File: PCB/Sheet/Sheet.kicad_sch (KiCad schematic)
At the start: 15 parts, among them U1 MCP9700Ax-ELT, U2 MCP2562-E-MF, U3 ATtiny1616-M, U6 MCP2515-xST

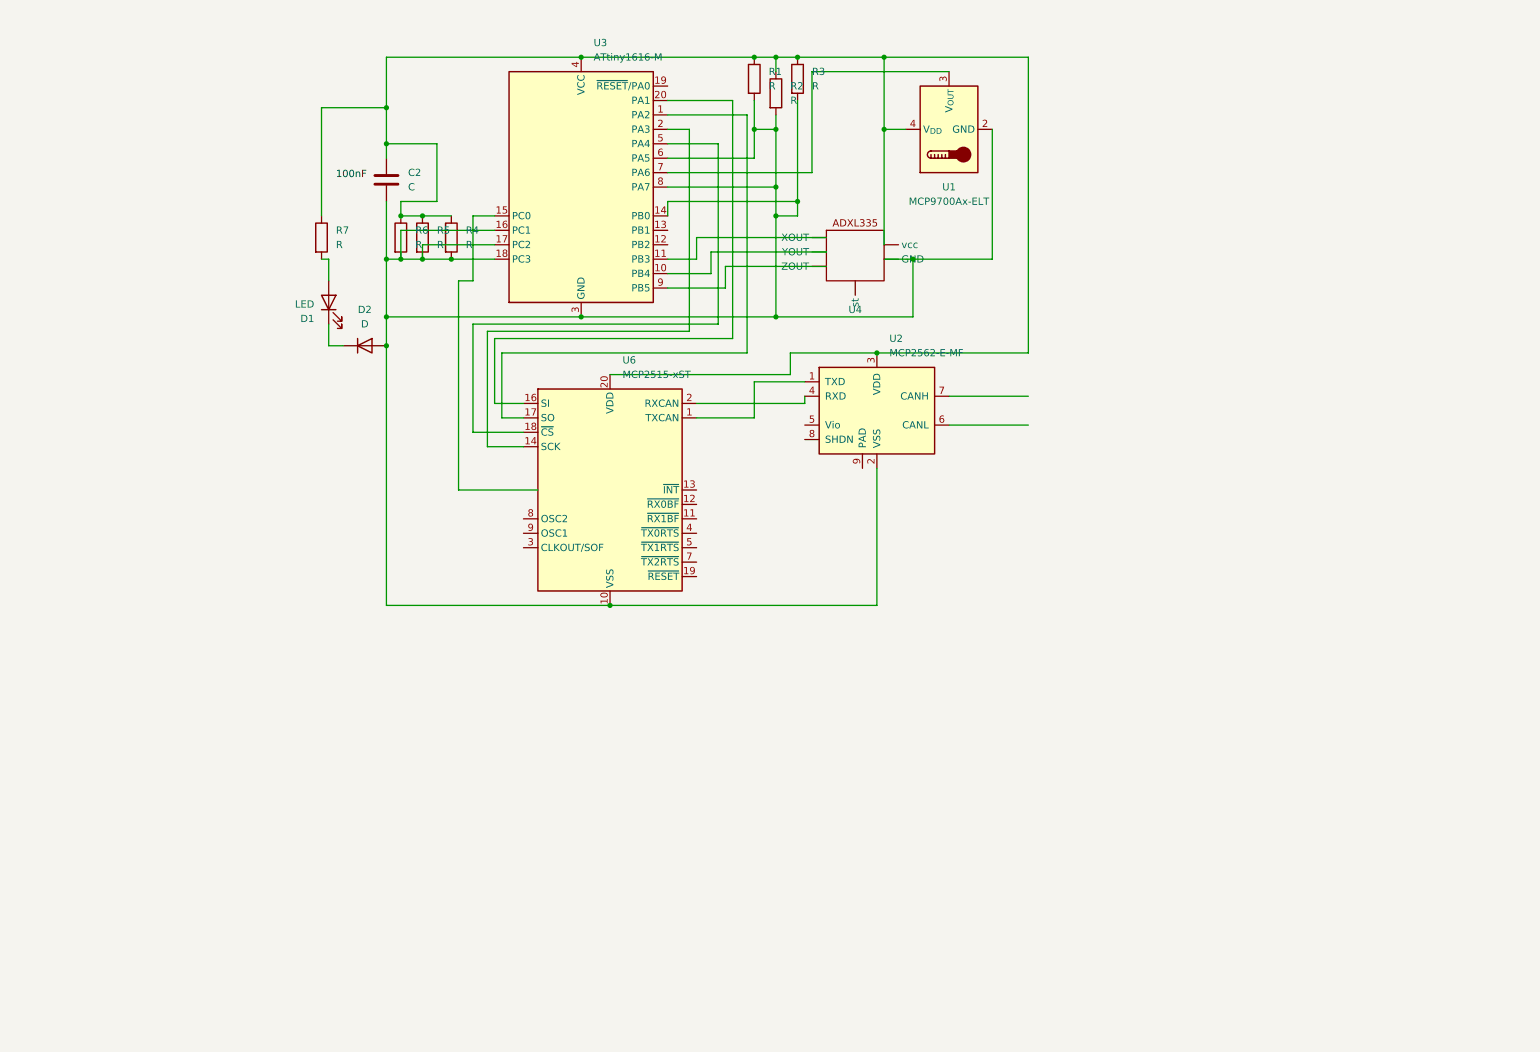
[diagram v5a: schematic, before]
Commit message: updates
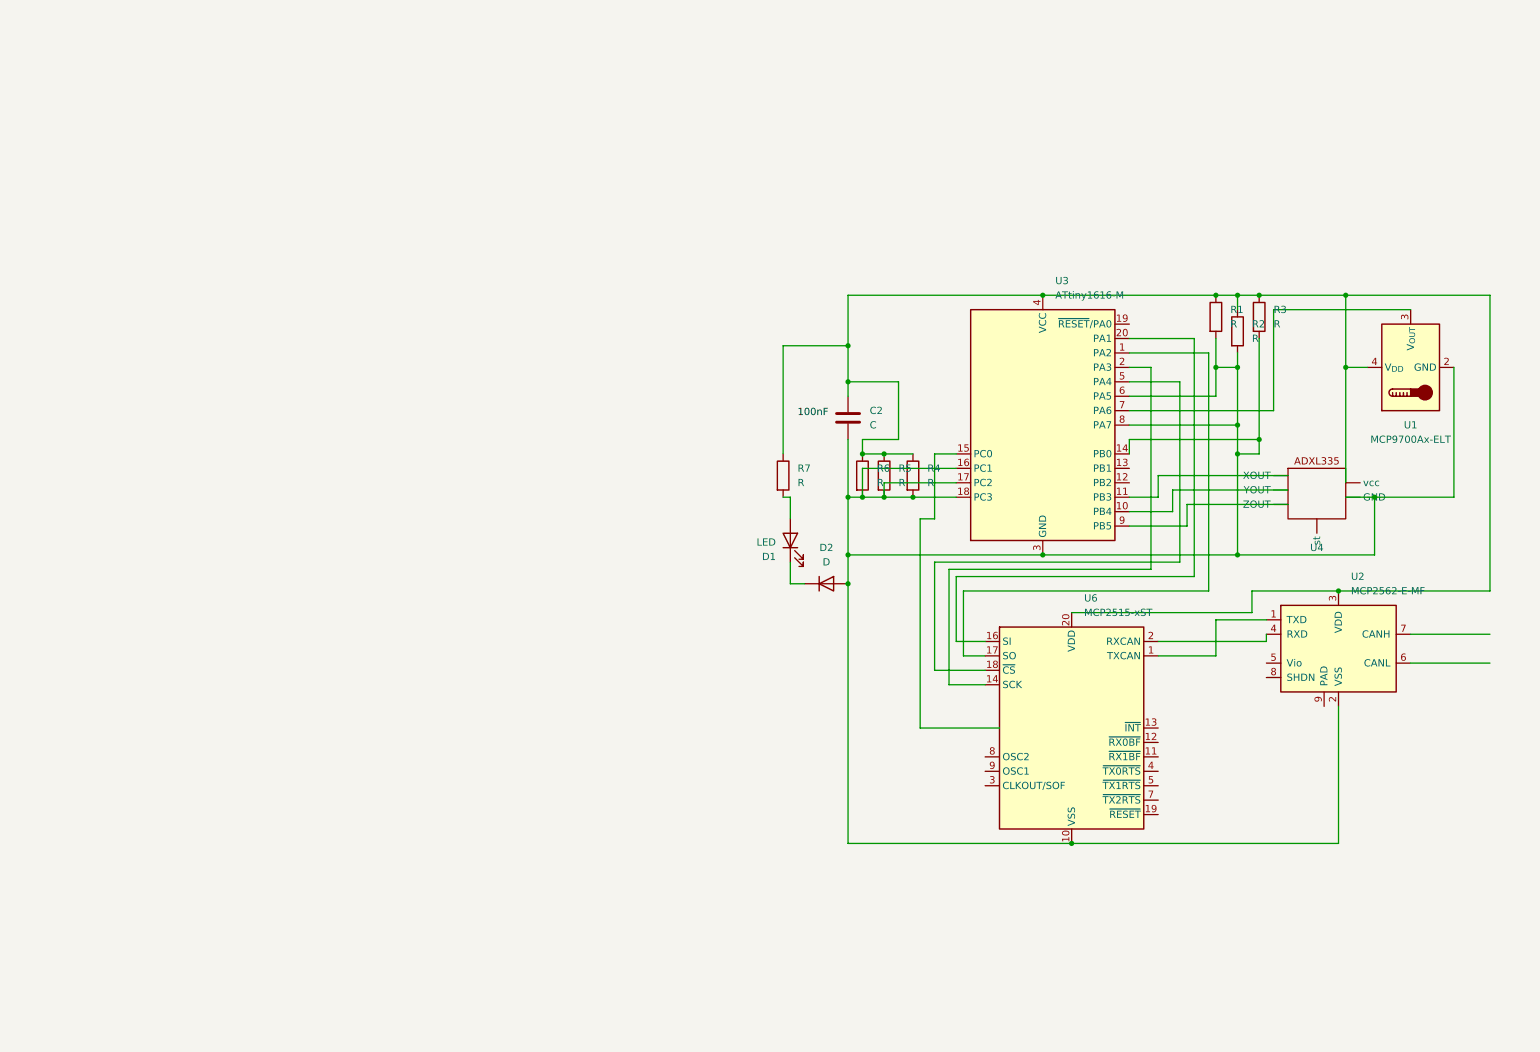
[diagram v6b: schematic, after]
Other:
- moved on the sheet: C2, D1, D2, R1, R2, R3, R4, R5, R6, R7, U1, U2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
